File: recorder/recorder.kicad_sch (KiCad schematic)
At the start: 13 parts, among them J1 GPIO_Conn_02x20_Odd_Even, U10 TPS7A4700RGWT, U2 ADAU7118

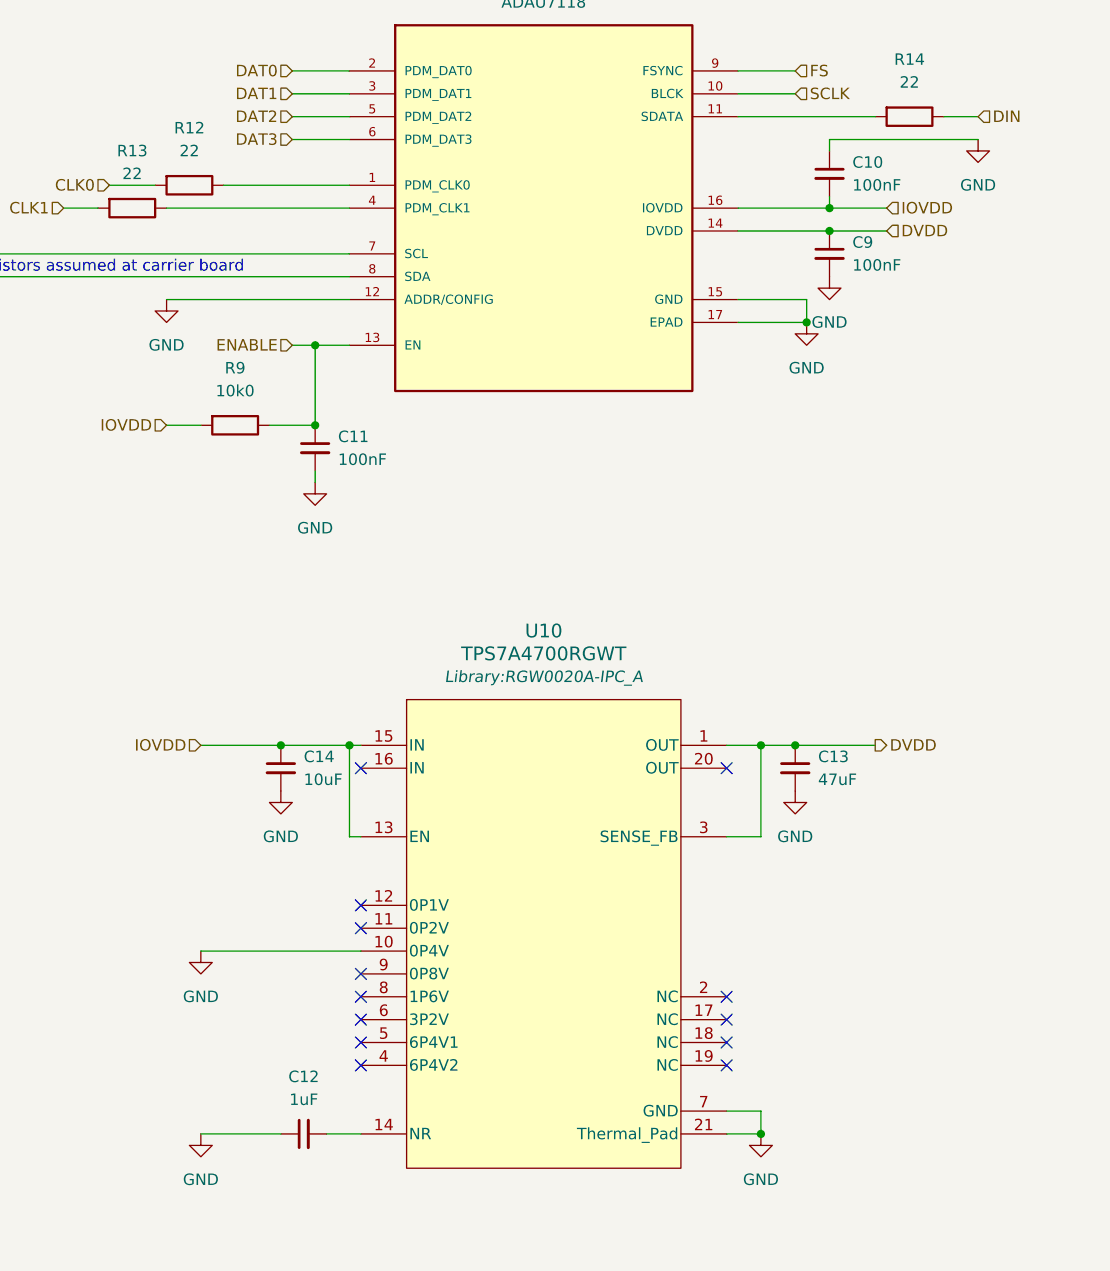
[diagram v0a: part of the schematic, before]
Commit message: MPN and Package
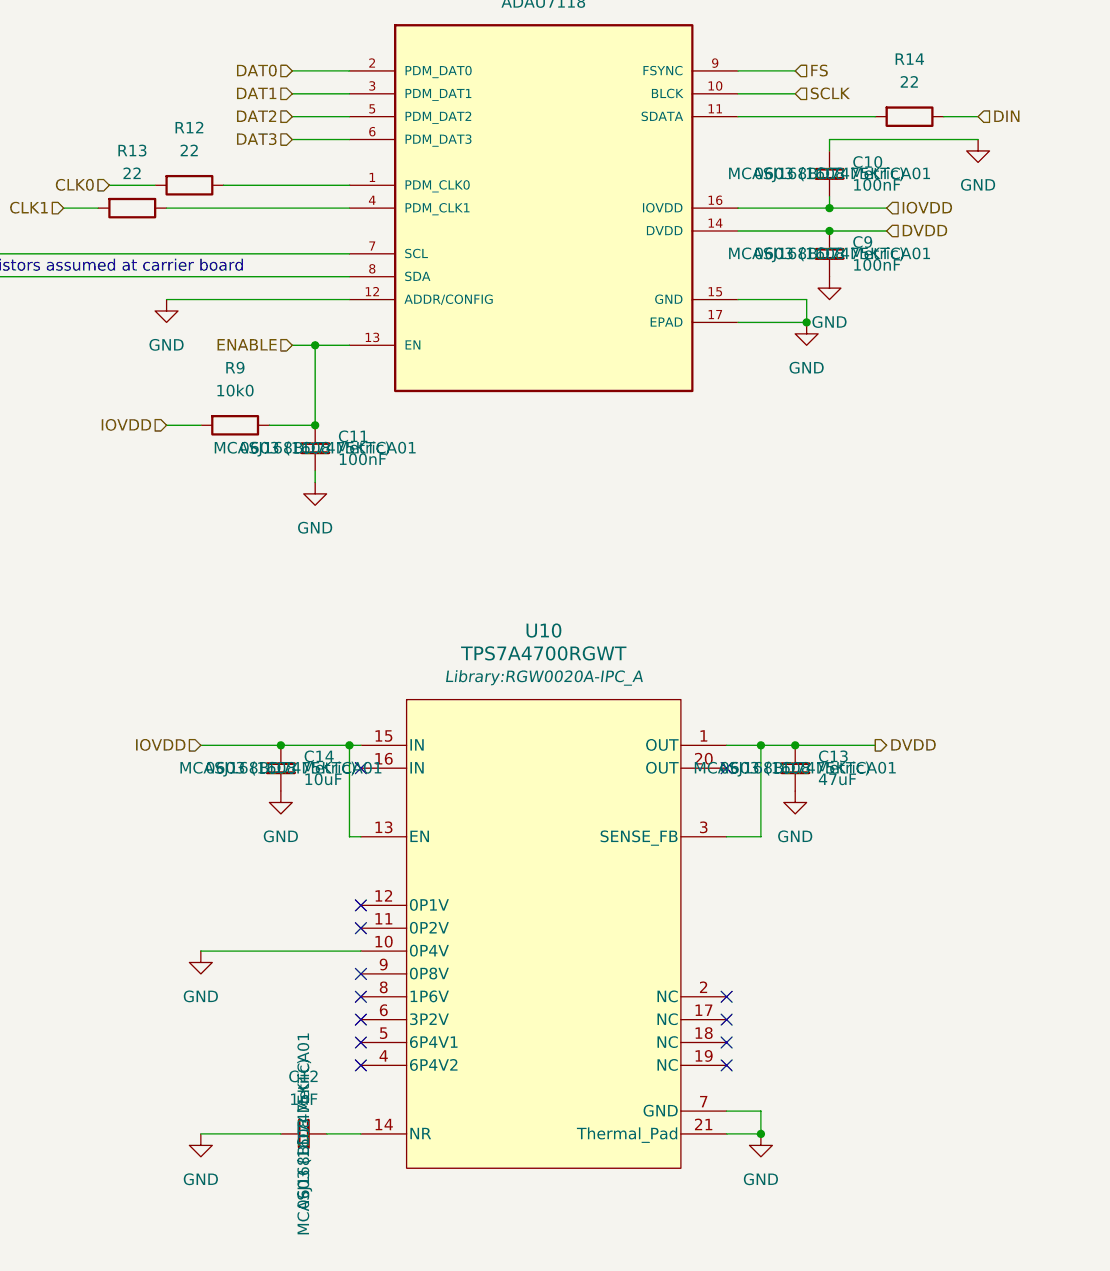
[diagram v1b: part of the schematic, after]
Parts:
- C10, C11, C12, C13, C14, C9: MPN (none) -> MCASJ168BD7475KTCA01; Package (none) -> 0603 (1608 Metric)
- J1: MPN (none) -> TSW-110-14-L-D; Manufacturer (none) -> Samtec; Package (none) -> 2x20 Pin Header, 2.54mm Pitch
- U10: MPN (none) -> TPS7A4700RGWT; Manufacturer (none) -> Texas Instruments; Package (none) -> VQFN-20
- U2: Availability Not in stock -> (none); Check_prices https://www.snapeda.com/parts/ADAU7118/Analog+Devices/view-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 -> (none); MF Analog Devices -> (none); MPN (none) -> ADAU7118ACPZRL; Manufacturer (none) -> Analog Devices; Package None -> LFCSP-16; Price None -> (none); SnapEDA_Link https://www.snapeda.com/parts/ADAU7118/Analog+Devices/view-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 -> (none)
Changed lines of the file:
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@@
+			)
+		)
+		(property "MPN" "MCASJ168BD7475KTCA01"
+			(at 77.47 104.14 0)
+			(effects
+				(font
+					(size 1.27 1.27)
+				)
+			)
+		)
+		(property "Package" "0603 (1608 Metric)"
+			(at 77.47 104.14 0)
+			(effects
+				(font
+					(size 1.27 1.27)
+				)
 			)
 		)
@@
 			)
 		)
+		(property "MPN" "TSW-110-14-L-D"
+			(at 214.63 82.55 0)
+			(effects
+				(font
+					(size 1.27 1.27)
+				)
+				(hide yes)
+			)
+		)
+		(property "Manufacturer" "Samtec"
+			(at 214.63 82.55 0)
+			(effects
+				(font
+					(size 1.27 1.27)
+				)
+				(hide yes)
+			)
+		)
+		(property "Package" "2x20 Pin Header, 2.54mm Pitch"
+			(at 214.63 82.55 0)
+			(effects
+				(font
+					(size 1.27 1.27)
+				)
+				(hide yes)
+			)
+		)
 		(pin "37"
 		)
@@
 			)
 		)
+		(property "MPN" "MCASJ168BD7475KTCA01"
+			(at 130.81 139.7 0)
+			(effects
+				(font
+					(size 1.27 1.27)
+				)
+			)
+		)
+		(property "Package" "0603 (1608 Metric)"
+			(at 130.81 139.7 0)
+			(effects
+				(font
+					(size 1.27 1.27)
+				)
+			)
+		)
 		(pin "1"
 		)
@@
 			)
 		)
+		(property "MPN" "MCASJ168BD7475KTCA01"
+			(at 134.62 73.66 0)
+			(effects
+				(font
+					(size 1.27 1.27)
+				)
+			)
+		)
+		(property "Package" "0603 (1608 Metric)"
+			(at 134.62 73.66 0)
+			(effects
+				(font
+					(size 1.27 1.27)
+				)
+			)
+		)
 		(pin "1"
 		)
@@
 			)
 		)
+		(property "MPN" "MCASJ168BD7475KTCA01"
+			(at 134.62 82.55 0)
+			(effects
+				(font
+					(size 1.27 1.27)
+				)
+			)
+		)
+		(property "Package" "0603 (1608 Metric)"
+			(at 134.62 82.55 0)
+			(effects
+				(font
+					(size 1.27 1.27)
+				)
+			)
+		)
 		(pin "2"
 		)
@@
 			)
 		)
+		(property "Package" "VQFN-20"
+			(at 82.55 137.16 0)
+			(effects
+				(font
+					(size 1.27 1.27)
+				)
+				(hide yes)
+			)
+		)
+		(property "MPN" "TPS7A4700RGWT"
+			(at 82.55 137.16 0)
+			(effects
+				(font
+					(size 1.27 1.27)
+				)
+				(hide yes)
+			)
+		)
+		(property "Manufacturer" "Texas Instruments"
+			(at 82.55 137.16 0)
+			(effects
+				(font
+					(size 1.27 1.27)
+				)
+				(hide yes)
+			)
+		)
 		(pin "13"
 		)
@@
 			)
 		)
+		(property "MPN" "MCASJ168BD7475KTCA01"
+			(at 73.66 139.7 0)
+			(effects
+				(font
+					(size 1.27 1.27)
+				)
+			)
+		)
+		(property "Package" "0603 (1608 Metric)"
+			(at 73.66 139.7 0)
+			(effects
+				(font
+					(size 1.27 1.27)
+				)
+			)
+		)
 		(pin "2"
 		)
@@
 			)
 		)
-		(property "MF" "Analog Devices"
+		(property "Manufacturer" "Analog Devices"
 			(at 104.14 74.93 0)
 			(effects
@@
 			)
 		)
-		(property "Package" "None"
-			(at 104.14 74.93 0)
-			(effects
-				(font
-					(size 1.27 1.27)
-				)
-				(justify bottom)
-				(hide yes)
-			)
-		)
-		(property "Price" "None"
-			(at 104.14 74.93 0)
-			(effects
-				(font
-					(size 1.27 1.27)
-				)
-				(justify bottom)
-				(hide yes)
-			)
-		)
-		(property "SnapEDA_Link" "https://www.snapeda.com/parts/ADAU7118/Analog+Devices/view-part/?ref=snap"
+		(property "Package" "LFCSP-16"
 			(at 104.14 74.93 0)
 			(effects
@@
 			)
 		)
-		(property "Availability" "Not in stock"
+		(property "MPN" "ADAU7118ACPZRL"
 			(at 104.14 74.93 0)
 			(effects
@@
 					(size 1.27 1.27)
 				)
-				(justify bottom)
-				(hide yes)
-			)
-		)
-		(property "Check_prices" "https://www.snapeda.com/parts/ADAU7118/Analog+Devices/view-part/?ref=eda"
-			(at 104.14 74.93 0)
-			(effects
-				(font
-					(size 1.27 1.27)
-				)
-				(justify bottom)
 				(hide yes)
 			)
@@
 			)
 		)
+		(property "MPN" "MCASJ168BD7475KTCA01"
+			(at 76.2 180.34 0)
+			(effects
+				(font
+					(size 1.27 1.27)
+				)
+			)
+		)
+		(property "Package" "0603 (1608 Metric)"
+			(at 76.2 180.34 0)
+			(effects
+				(font
+					(size 1.27 1.27)
+				)
+			)
+		)
